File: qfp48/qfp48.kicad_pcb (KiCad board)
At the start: 2 copper layers, 25.4 x 63.5 mm, 5 parts, among them J1 Conn_01x24_Pin, J2 Conn_01x24_Pin, U1 STM32G0B0CETx

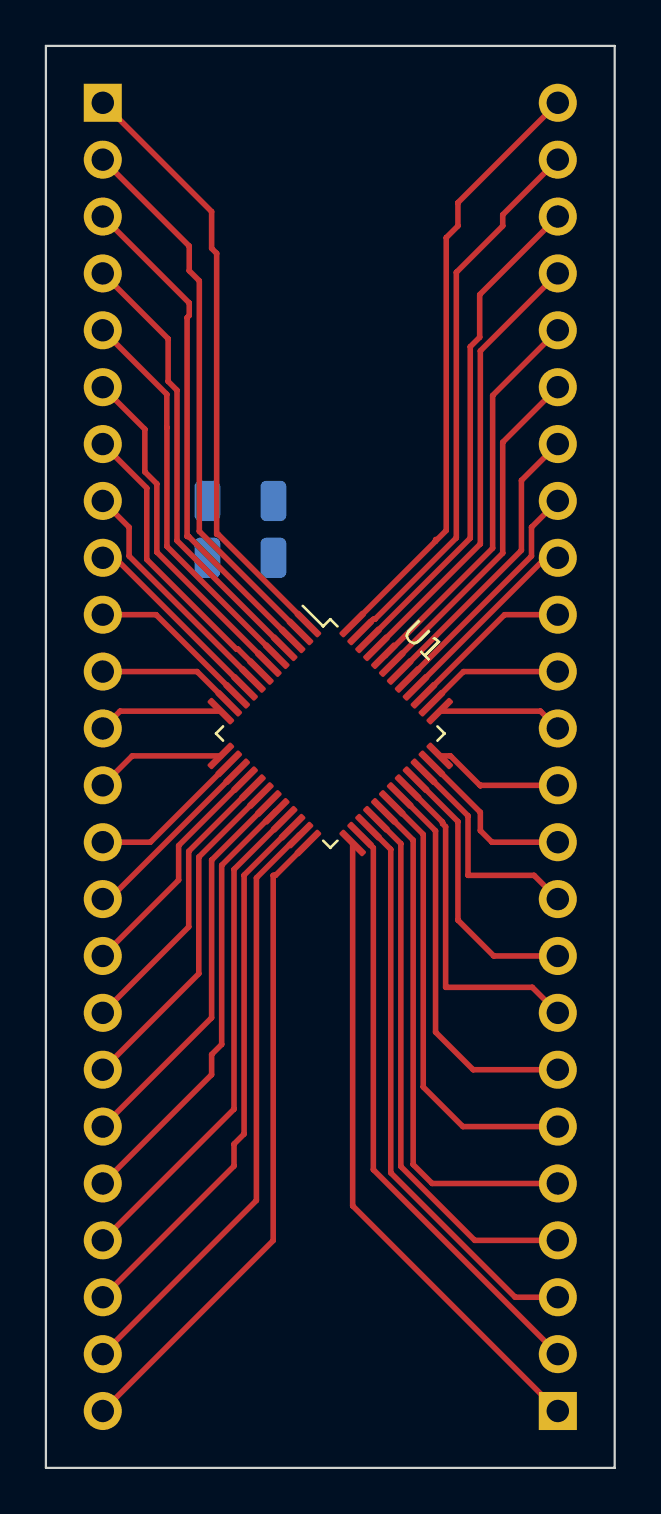
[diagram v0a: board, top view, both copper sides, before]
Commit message: Finish - order in PCBWAY
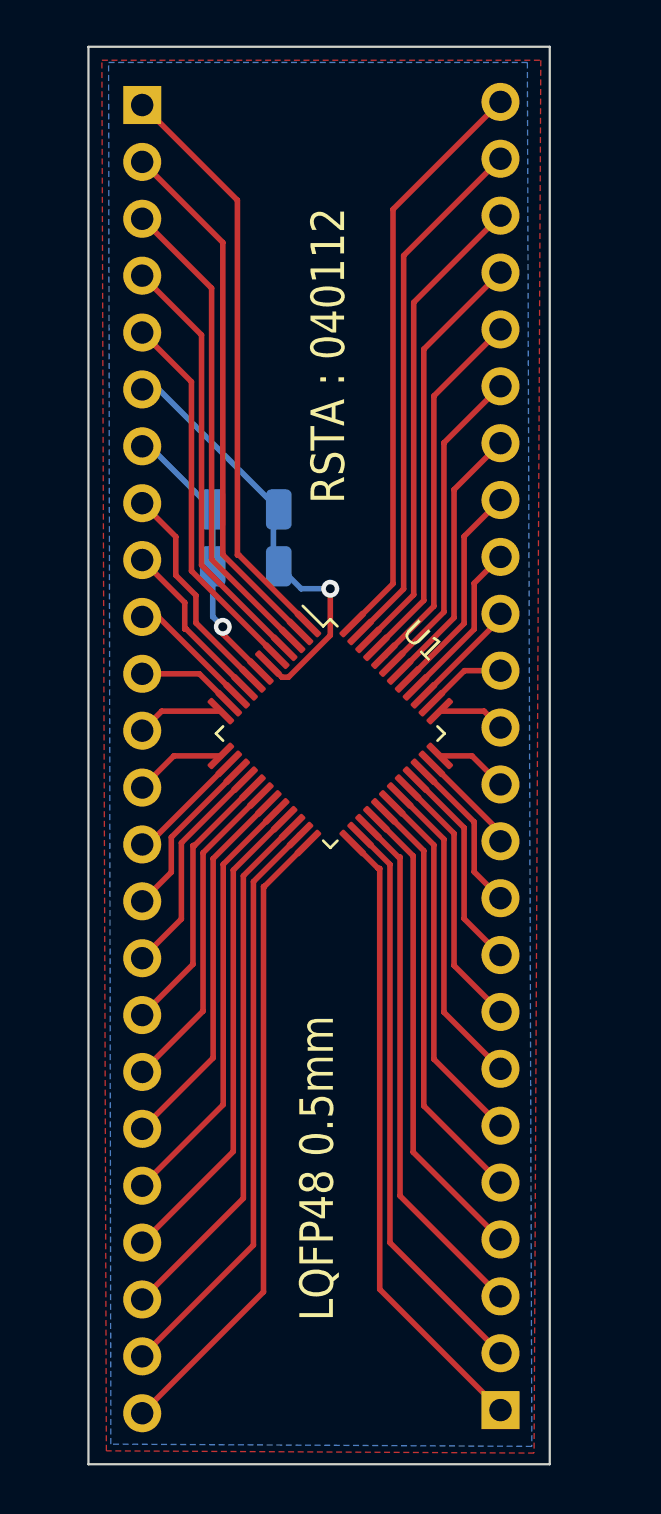
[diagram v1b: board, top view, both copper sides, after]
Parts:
- moved C1 2.93 mm to (110.5, 84.2), turned to 180 degrees
- moved J2 2.56 mm to (121.9, 121.9)
- moved C2 2.17 mm to (110.5, 81.7), turned to 180 degrees
- moved J1 1.76 mm to (105.9, 63.6)
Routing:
- net Net-(J2-Pin_5): track 23.1 -> 18.7 mm
- net VDD: track 15.4 -> 19.5 mm, vias 0 -> 1
- net Net-(J2-Pin_6): track 20.0 -> 16.4 mm
- net Net-(J2-Pin_8): track 15.1 -> 11.7 mm
- net Net-(J2-Pin_7): track 17.4 -> 14.1 mm
- net Net-(J2-Pin_4): track 24.3 -> 21.1 mm
- net Net-(J2-Pin_10): track 9.89 -> 7.06 mm
- net Net-(J2-Pin_11): track 7.55 -> 4.73 mm
- net Net-(J2-Pin_9): track 12.2 -> 9.40 mm
- net Net-(J2-Pin_12): track 5.83 -> 3.24 mm
- net Net-(J2-Pin_13): track 5.59 -> 3.02 mm
- net Net-(J2-Pin_14): track 6.21 -> 3.67 mm
- net Net-(J2-Pin_15): track 7.47 -> 5.06 mm
- net Net-(J2-Pin_3): track 25.6 -> 23.4 mm
- net Net-(J1-Pin_11): track 6.21 -> 4.41 mm
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- added copper zone on B.Cu, net GND
- added copper zone on F.Cu, net VDD
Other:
- board size 25.4 x 63.5 mm -> 20.6 x 63.3 mm
- board text added: "LQFP48 0.5mm"
- board text added: "RSTA : 040112"
